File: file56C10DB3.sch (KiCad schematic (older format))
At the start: 31 parts, among them P1 BL_PAD, P10 CONN_01X01, P2 SWD_DAT, P3 SWD_CLK, P4 SWD_3V3, P5 SWD_GND, P6 SWD_RST, P7 CONN_01X01, P8 CONN_01X01, P9 CONN_01X01, U5 SAMD21E17A, Y1 32.768kHz

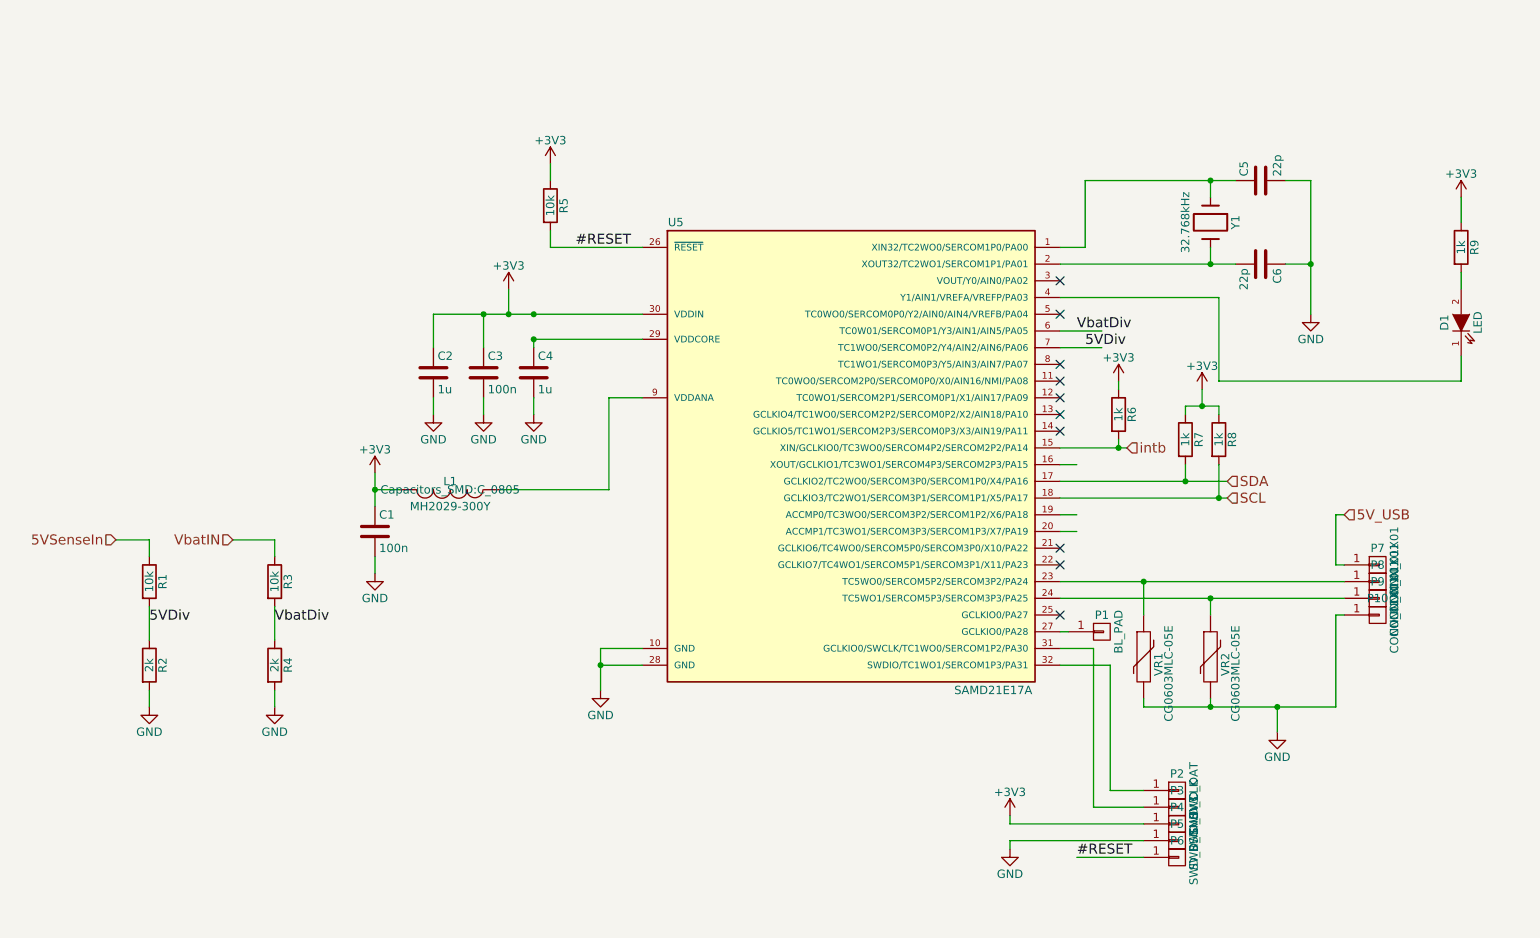
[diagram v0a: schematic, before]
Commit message: started layout, completed schematic
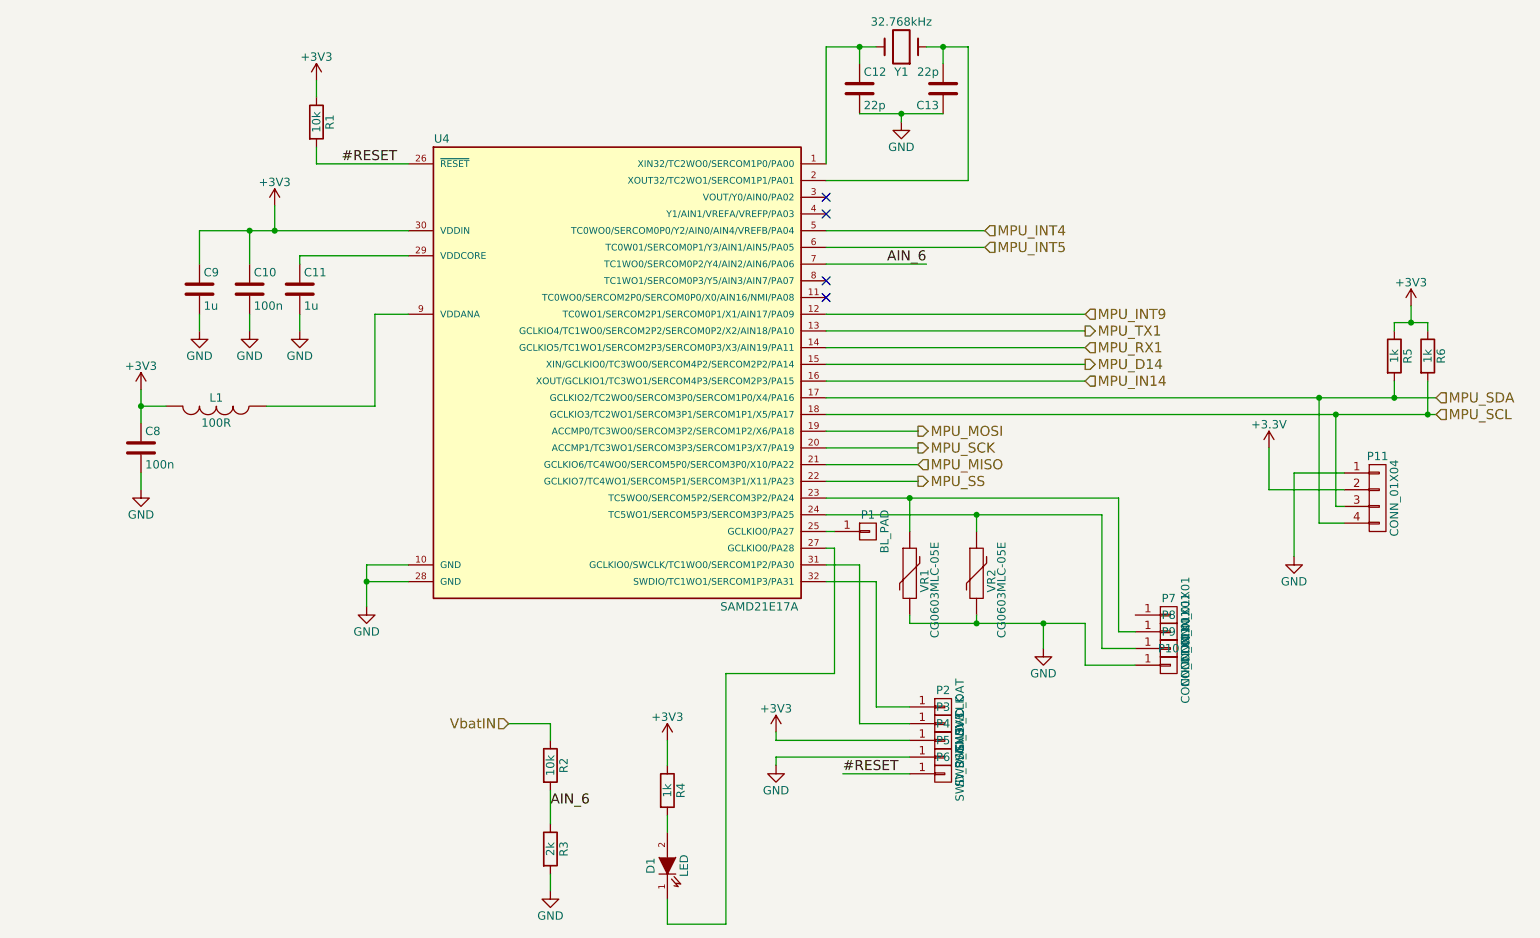
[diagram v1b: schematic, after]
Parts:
- removed R1: 10k, Capacitors_SMD:C_0603, symbol R
- removed R2: 2k, Capacitors_SMD:C_0603, symbol R
- removed R6: 1k, Capacitors_SMD:C_0603, symbol R
- added P11: CONN_01X04, symbol CONN_01X04
- L1: value MH2029-300Y -> 100R; footprint Capacitors_SMD:C_0805 -> ~
- renumbered C3 to C10, C4 to C11, C5 to C12, C6 to C13, C1 to C8, C2 to C9, R5 to R1, R3 to R2, R4 to R3, R9 to R4, R7 to R5, R8 to R6, U5 to U4
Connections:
- net labels added: +3.3V, AIN_6, MPU_D14, MPU_IN14, MPU_INT4, MPU_INT5, MPU_INT9, MPU_MISO, MPU_MOSI, MPU_RX1, MPU_SCK, MPU_SCL, MPU_SDA, MPU_SS, MPU_TX1
- net labels removed: 5VDiv, 5VSenseIn, 5V_USB, SCL, SDA, VbatDiv, intb
- wire segments 85 -> 96
- no-connect marks 10 -> 4
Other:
- moved on the sheet: C10, C11, C12, C13, C8, C9, D1, L1, P1, P10, P2, P3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
